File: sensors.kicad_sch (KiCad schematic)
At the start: 27 parts, among them U2 LIS2DH12TR, U3 L3GD20HTR, U4 MP6515GF-Z, U5 MP6515GF-Z, U6 MP6515GF-Z, U7 DRV5055A4xLPGxQ1, U8 DRV5055A4xLPGxQ1, U9 DRV5055A4xLPGxQ1

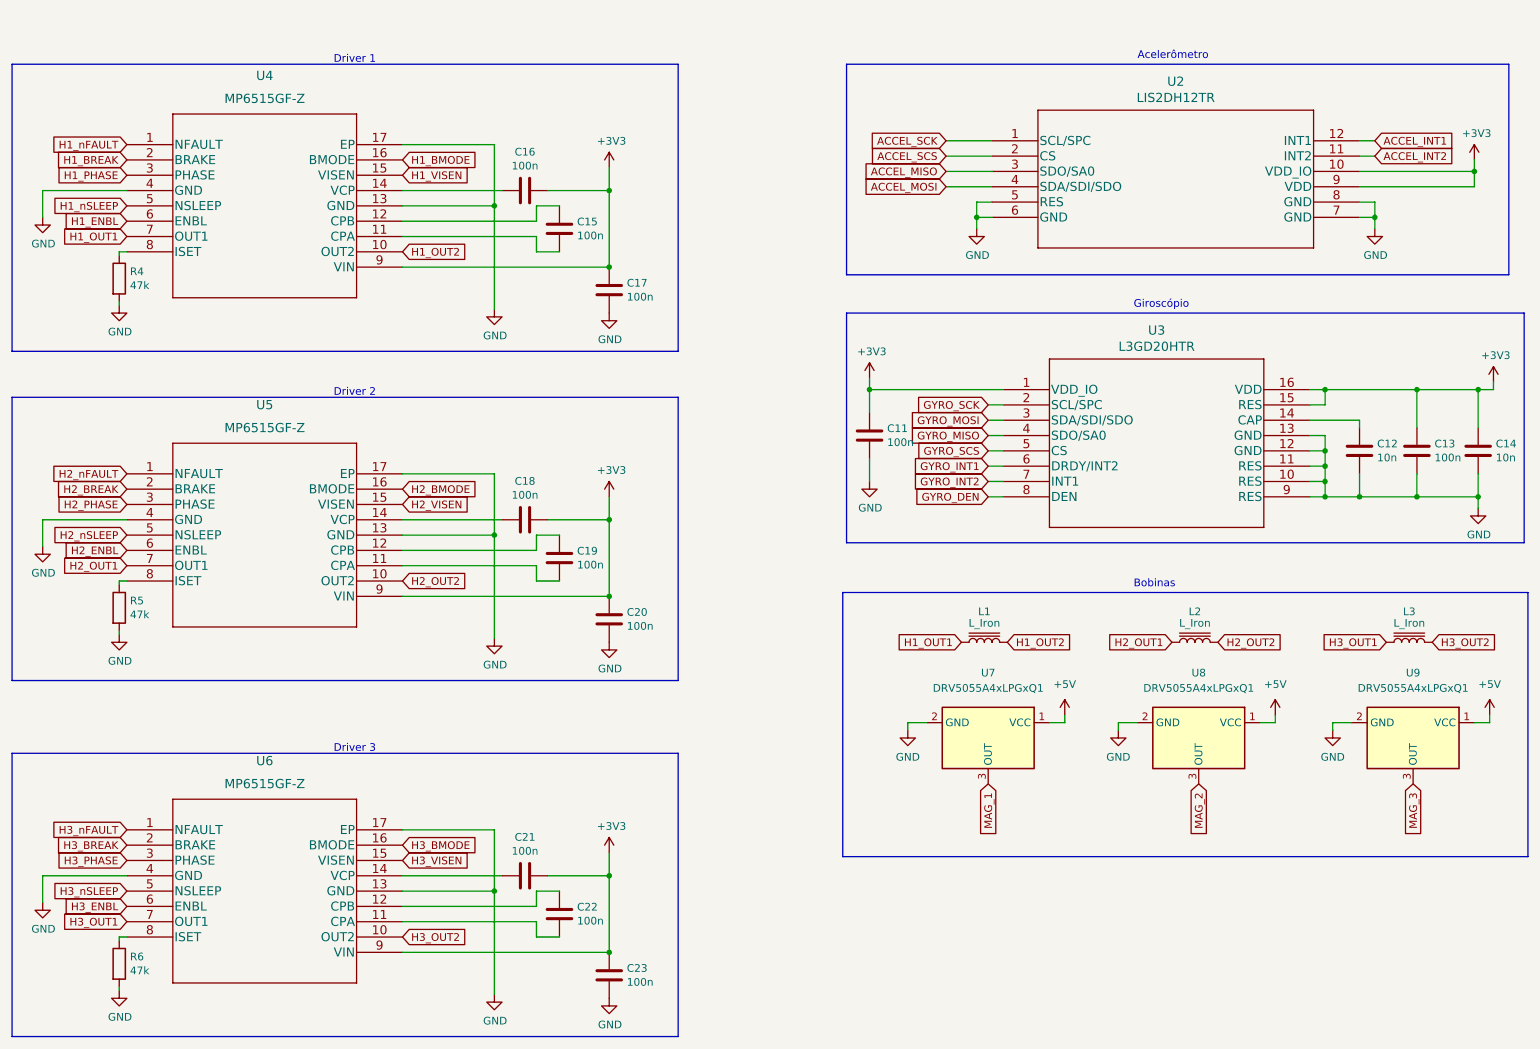
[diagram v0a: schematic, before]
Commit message: last commit
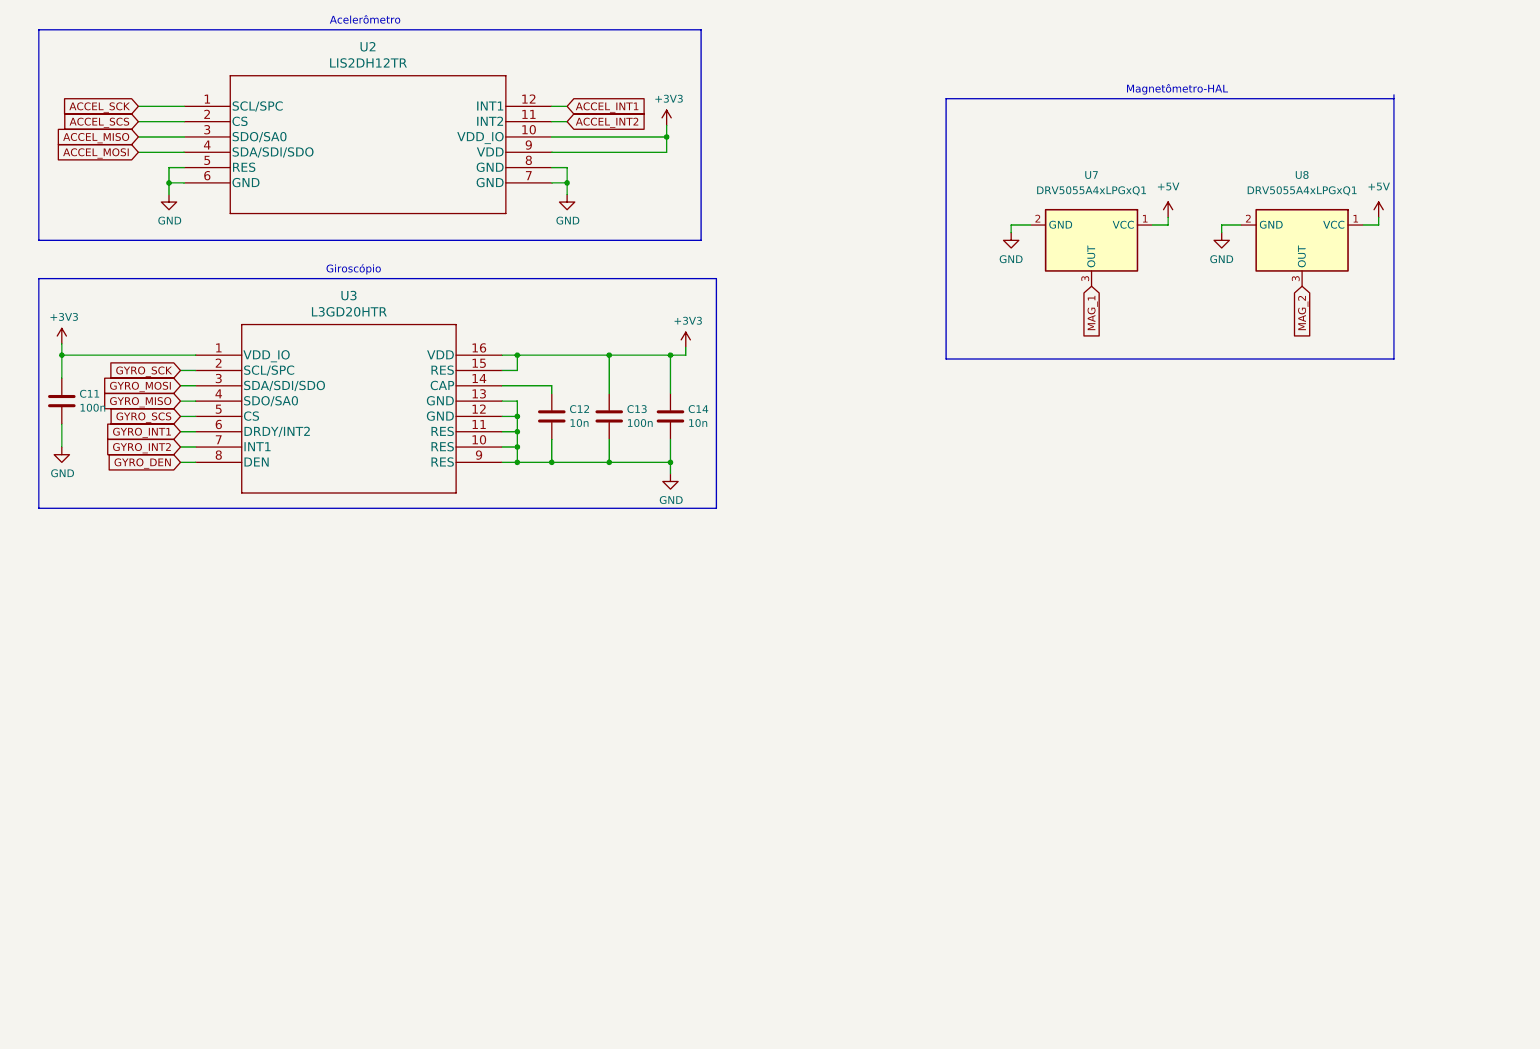
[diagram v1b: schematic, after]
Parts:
- removed C15, C16, C17, C18, C19, C20, C21, C22, C23: 100n, Capacitor_SMD:C_0805_2012Metric, symbol Device:C
- removed L1, L2, L3: L_Iron, magnetorque_lib:magnetorquer, symbol Device:L_Iron
- removed R4, R5, R6: 47k, Resistor_SMD:R_0805_2012Metric, symbol Device:R
- removed U4, U5, U6: MP6515GF-Z, magnetorque_lib:MP6515GF-Z, symbol mp65:MP6515GF-Z
- removed U9: DRV5055A4xLPGxQ1, Package_TO_SOT_THT:TO-92_Inline, symbol Sensor_Magnetic:DRV5055A4xLPGxQ1
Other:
- note added: "Magnetômetro-HAL"
- note removed: "Bobinas"
- note removed: "Driver 1"
- note removed: "Driver 2"
- note removed: "Driver 3"
- moved on the sheet: C11, C12, C13, C14, U2, U3, U7, U8
